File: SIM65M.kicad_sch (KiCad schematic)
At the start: 24 parts, among them J1 Conn_01x11_Pin, J2 U.FL-R-SMT_10_, Q1 AO3400A, Q2 DTC143ZUAT106, Q3 DTC143ZUAT106, U1 SIM65M_C7495025, U2 BWGNSCNX25-25W4, U5 XC6206P282MR-G

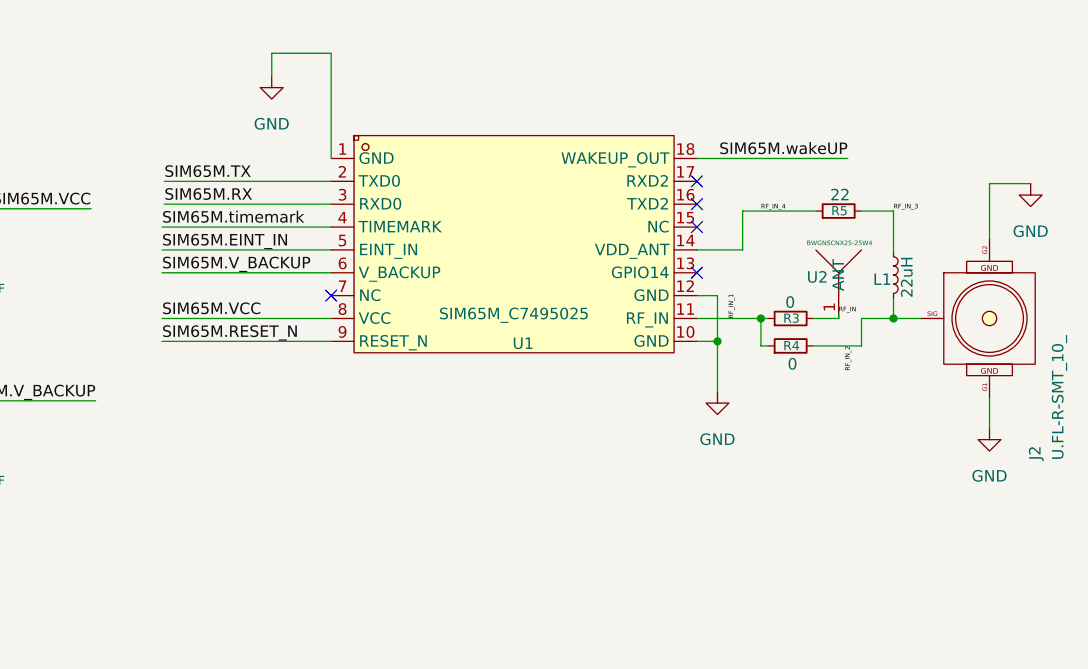
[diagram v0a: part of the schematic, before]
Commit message: carga
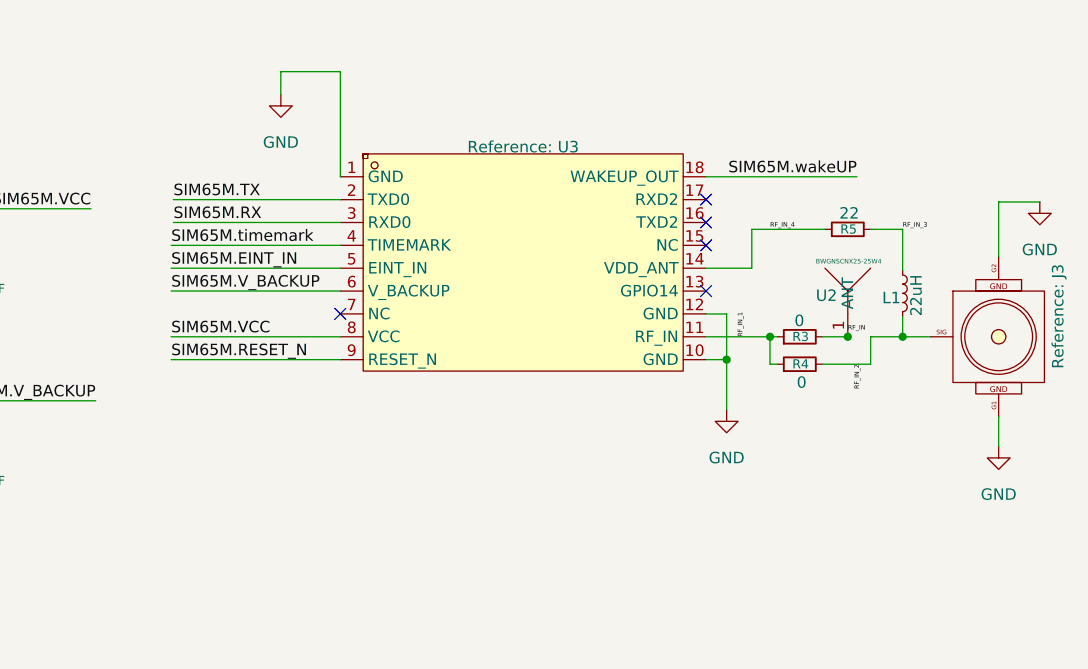
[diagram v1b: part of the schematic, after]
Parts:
- removed J2: U.FL-R-SMT_10_, Snapeda:U.FL-R-SMT_10_-foot, symbol Snapeda:U.FL-R-SMT_10_
- removed U1: SIM65M_C7495025, Snapeda:SIM65M_foot, symbol Snapeda:SIM65M_C7495025
- added J3: U.FL-R-SMT_10_, Snapeda:U.FL-R-SMT_10_-foot, symbol Snapeda:U.FL-R-SMT_10_
- added U3: SIM65M_C7495025, Snapeda:SIM65M_foot, symbol Snapeda:SIM65M_C7495025
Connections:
- net GND: now also J3.G1, J3.G2, U3.1 (GND), U3.10 (GND), U3.12 (GND)
- net PIN.V_BACKUP: now also U3.6 (V_BACKUP)
- net RF_IN_1: now also U3.11 (RF_IN)
- net RF_IN_2: now also J3.SIG
- net RF_IN_4: now also U3.14 (VDD_ANT)
- net SIM65M.EINT_IN: now also U3.5 (EINT_IN)
- net SIM65M.RESET_N: now also U3.9 (RESET_N)
- net SIM65M.RX: now also U3.3 (RXD0)
- net SIM65M.TX: now also U3.2 (TXD0)
- net SIM65M.VCC: now also U3.8 (VCC)
- net SIM65M.timemark: now also U3.4 (TIMEMARK)
- net SIM65M.wakeUP: now also U3.18 (WAKEUP_OUT)
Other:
- moved on the sheet: L1, R3, R4, R5, U2
